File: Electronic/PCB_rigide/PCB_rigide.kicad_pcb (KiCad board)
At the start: 2 copper layers, 24 parts, among them J1 Conn_01x02_Pin, J2 Conn_01x04_Socket, J3 Conn_01x01_Socket, J4 Conn_01x01_Socket, J5 Conn_01x01_Socket, U2 BMA400, Y1 Crystal_GND24

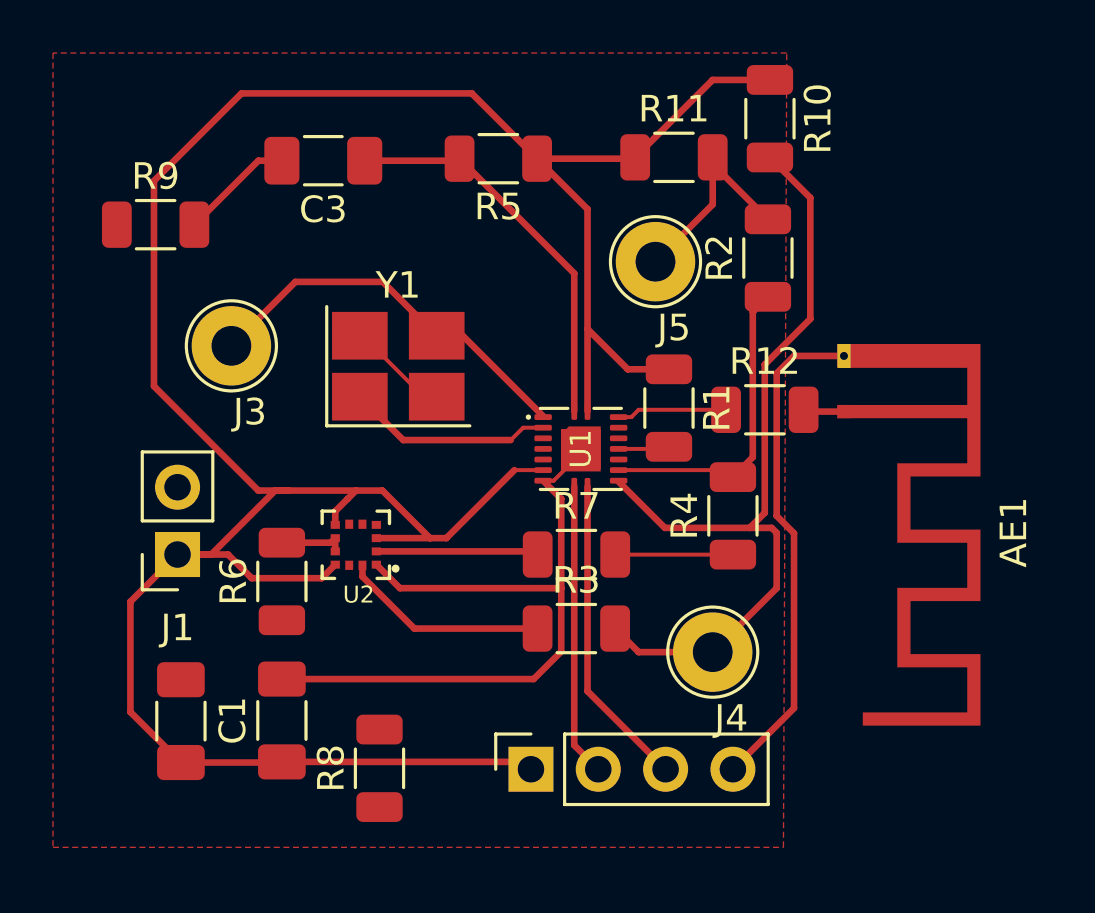
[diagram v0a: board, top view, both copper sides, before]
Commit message: update electronic
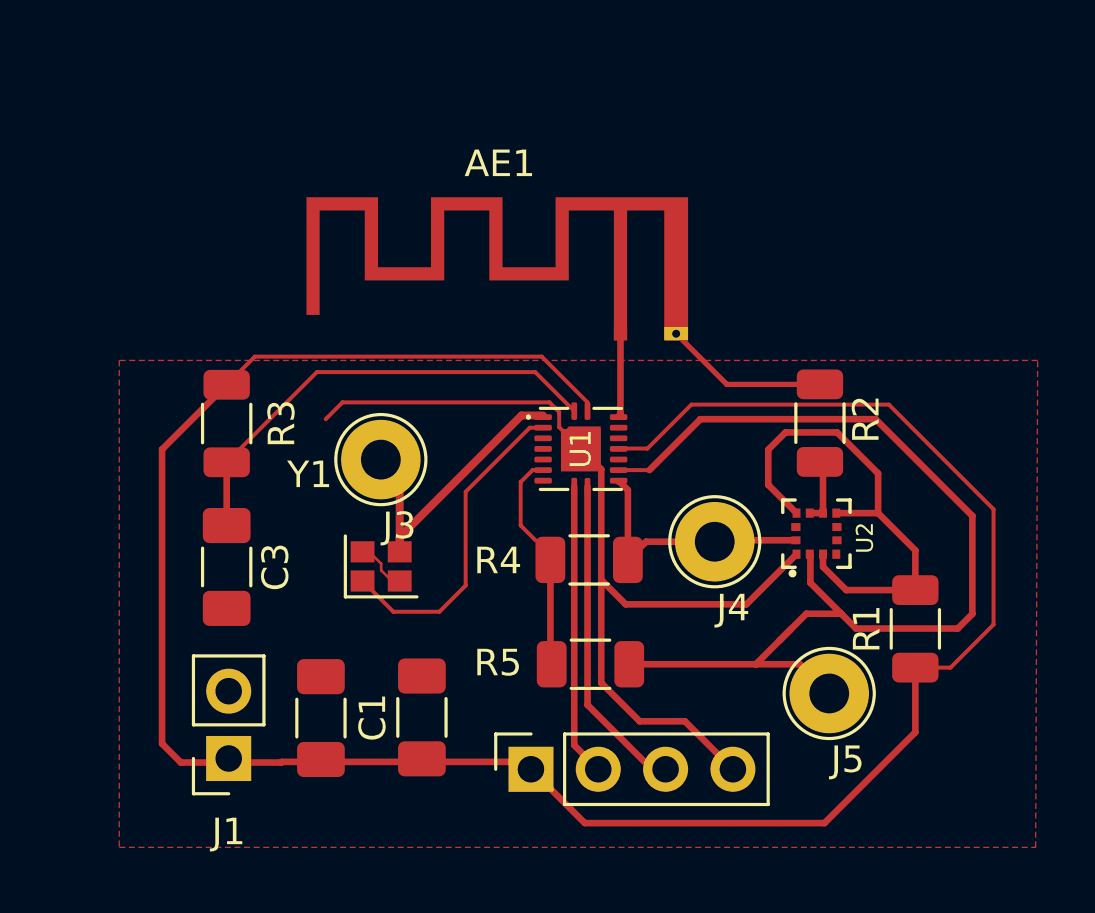
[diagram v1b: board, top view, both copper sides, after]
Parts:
- removed R12, R6, R7, R8, R9: 0, Resistor_SMD:R_1206_3216Metric
- removed the R3 at (96.7, 46.1)
- removed the R4 at (102.6, 41.8)
- AE1: footprint RF_Antenna:Texas_SWRA117D_2.4GHz_Right -> RF_Antenna:Texas_SWRA117D_2.4GHz_Left
- Y1: footprint Crystal:Crystal_SMD_3225-4Pin_3.2x2.5mm_HandSoldering -> Crystal:Crystal_SMD_2016-4Pin_2.0x1.6mm
- moved R5 19.4 mm to (97.2, 47.4)
- moved R4 18.0 mm to (97.2, 43.5), turned to 0 degrees
- moved J5 17.6 mm to (106.2, 48.5)
- moved U2 17.4 mm to (105.8, 42.5), turned to 90 degrees
- moved C3 15.8 mm to (83.5, 43.8), turned to -90 degrees
- moved R3 14.3 mm to (83.5, 38.4), turned to -90 degrees
- moved R1 12.5 mm to (109.5, 46.1), turned to 90 degrees
- moved AE1 8.93 mm to (98.4, 35.0), turned to 0 degrees
- moved J1 7.93 mm to (83.6, 51.0)
- moved Y1 7.58 mm to (89.3, 43.8)
- moved J3 7.09 mm to (89.3, 39.7)
- moved R2 6.53 mm to (105.9, 38.4)
- moved C1 5.28 mm to (90.9, 49.5)
- moved C2 5.28 mm to (87.1, 49.5)
- moved J4 4.17 mm to (101.9, 42.8)
- renumbered R5 to R3, R10 to R4, R11 to R5
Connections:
- R2 pad 1: I2C_SDA -> GND
- R2 pad 2: I2C_SDA -> GND
- R4 pad 1: VCC -> SW0
- R5 pad 1: VCC -> SW0
- U1 pad 6: VCC -> SW0
- U1 pad 7: GND -> unconnected-(U1-SW1-Pad7)
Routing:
- net I2C_SCL: track 39.7 -> 9.49 mm
- net GND: track 58.5 -> 45.8 mm
- net I2C_SDA: track 30.4 -> 40.6 mm
- net SW0: track 0.00 -> 7.91 mm
- net XO_P: track 7.79 -> 12.2 mm
- net XO_N: track 14.9 -> 11.6 mm
- net RF_TX: track 6.11 -> 3.14 mm
- net Net-(U1-EN): track 14.9 -> 17.5 mm
